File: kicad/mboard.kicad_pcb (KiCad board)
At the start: 2 copper layers, 66 x 48.3 mm, 3 parts

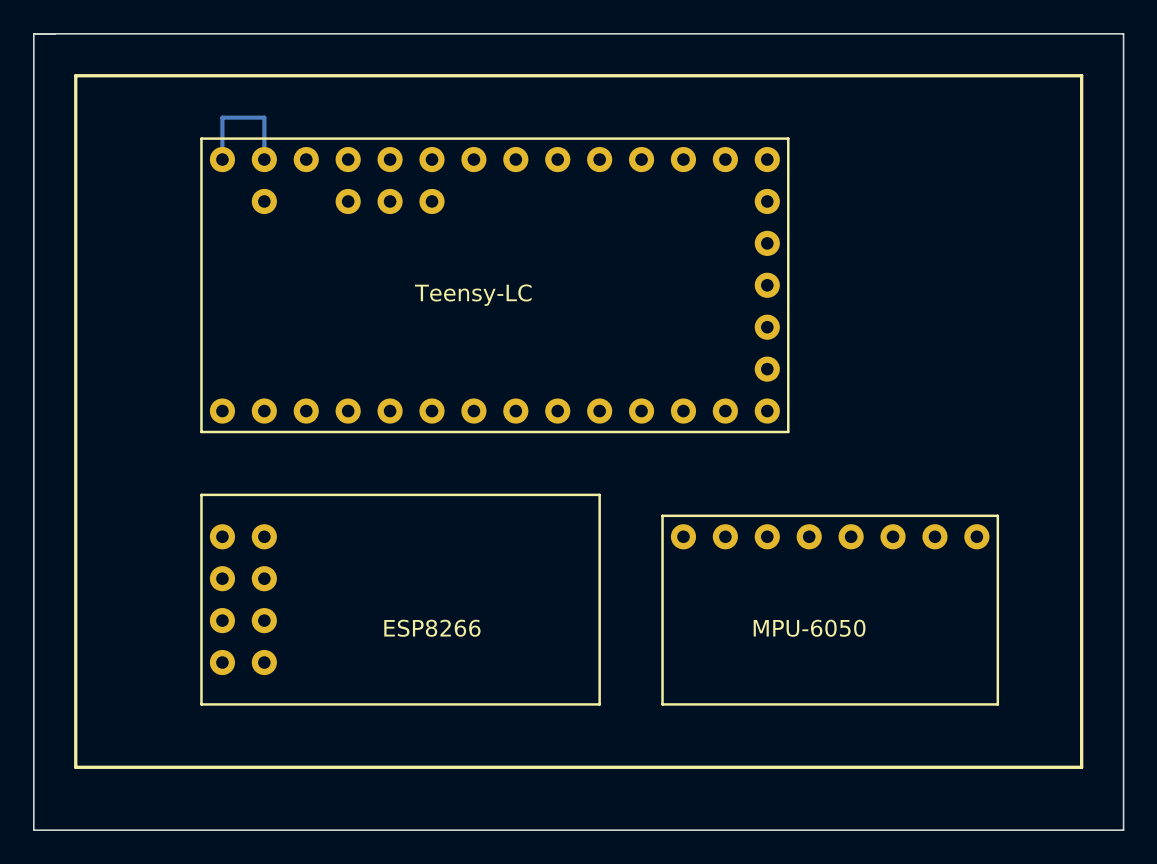
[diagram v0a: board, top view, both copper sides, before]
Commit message: mpu6050 thin
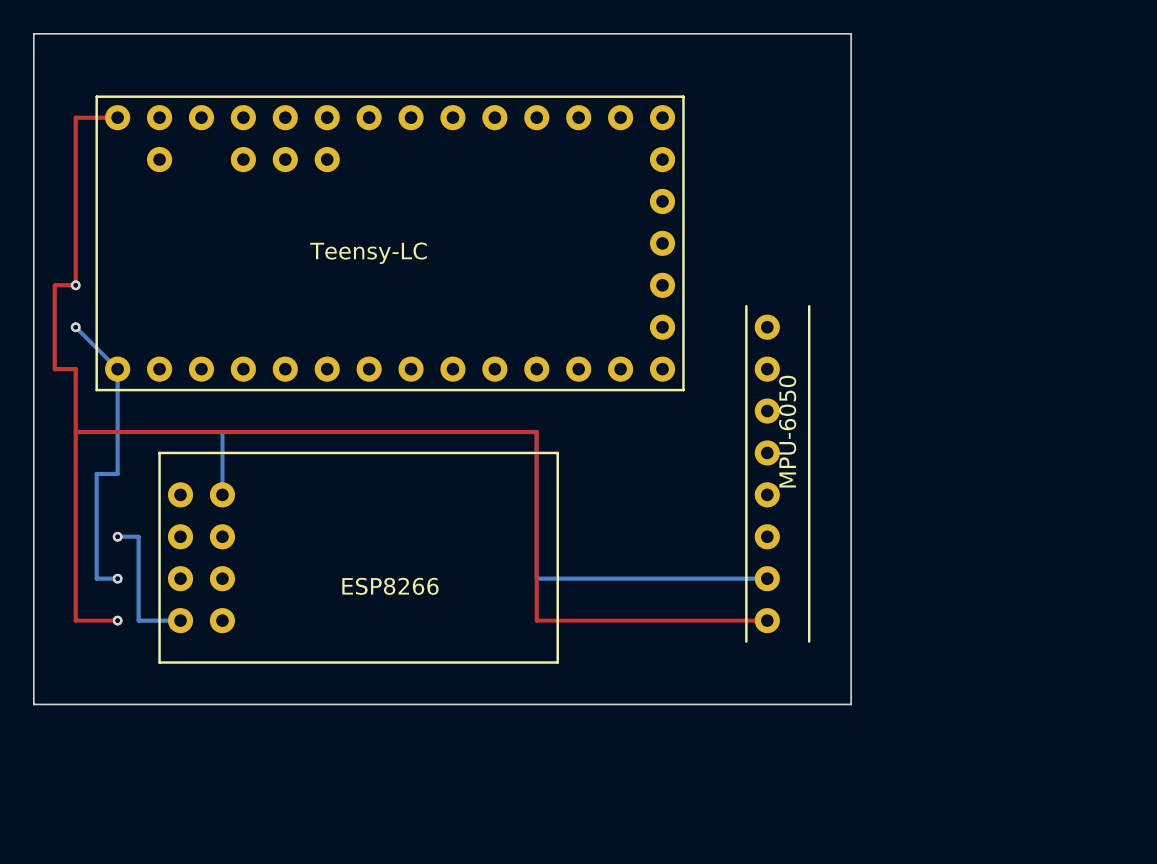
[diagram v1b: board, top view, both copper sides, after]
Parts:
- MPU-6050: footprint modules:MPU6050 -> modules:MPU6050-thin
- moved MPU-6050 8.03 mm to (74.9, 63.5), turned to 90 degrees
- moved Teensy-LC 6.84 mm to (45.7, 48.3)
- moved ESP8266 3.59 mm to (47.0, 68.6)
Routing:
- net (no net): track 7.62 -> 171.2 mm, vias 0 -> 5
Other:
- board size 66 x 48.3 mm -> 49.5 x 40.6 mm
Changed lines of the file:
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@@
     (links 0)
     (no_connects 0)
-    (area 25.349999 35.509999 91.490001 83.870001)
+    (area 25.349999 35.509999 74.980001 76.250001)
     (thickness 1.6)
-    (drawings 9)
-    (tracks 3)
+    (drawings 4)
+    (tracks 30)
     (zones 0)
     (modules 3)
@@
     (pad_to_mask_clearance 0)
     (aux_axis_origin 0 0)
-    (visible_elements FFFFFF7F)
+    (visible_elements FFFFF77F)
     (pcbplotparams
       (layerselection 0x010f0_80000001)
@@
   )
   (module modules:ESP8266 (layer F.Cu)
-    (at 49.53 71.12)
+    (at 46.99 68.58)
     (fp_text reference ESP8266 (at 0 0.5) (layer F.SilkS)
       (effects (font (size 1 1) (thickness 0.15)))
@@
     (pad 9 thru_hole circle (at -10.16 -5.08) (size 1.524 1.524) (drill 0.762) (layers *.Cu *.Mask F.SilkS))
   )
-  (module modules:MPU6050 (layer F.Cu)
-    (at 72.39 71.12)
-    (fp_text reference MPU-6050 (at 0 0.5) (layer F.SilkS)
-      (effects (font (size 1 1) (thickness 0.15)))
-    )
-    (fp_text value MPU6050 (at 0 -0.5) (layer F.Fab)
-      (effects (font (size 1 1) (thickness 0.15)))
-    )
-    (fp_line (start -8.89 -6.35) (end 11.43 -6.35) (layer F.SilkS) (width 0.15))
-    (fp_line (start 11.43 -6.35) (end 11.43 5.08) (layer F.SilkS) (width 0.15))
-    (fp_line (start 11.43 5.08) (end -8.89 5.08) (layer F.SilkS) (width 0.15))
-    (fp_line (start -8.89 5.08) (end -8.89 -6.35) (layer F.SilkS) (width 0.15))
-    (pad 1 thru_hole circle (at -7.62 -5.08) (size 1.524 1.524) (drill 0.762) (layers *.Cu *.Mask F.SilkS))
-    (pad 2 thru_hole circle (at -5.08 -5.08) (size 1.524 1.524) (drill 0.762) (layers *.Cu *.Mask F.SilkS))
-    (pad 3 thru_hole circle (at -2.54 -5.08) (size 1.524 1.524) (drill 0.762) (layers *.Cu *.Mask F.SilkS))
-    (pad 4 thru_hole circle (at 0 -5.08) (size 1.524 1.524) (drill 0.762) (layers *.Cu *.Mask F.SilkS))
-    (pad 5 thru_hole circle (at 2.54 -5.08) (size 1.524 1.524) (drill 0.762) (layers *.Cu *.Mask F.SilkS))
-    (pad 6 thru_hole circle (at 5.08 -5.08) (size 1.524 1.524) (drill 0.762) (layers *.Cu *.Mask F.SilkS))
-    (pad 7 thru_hole circle (at 7.62 -5.08) (size 1.524 1.524) (drill 0.762) (layers *.Cu *.Mask F.SilkS))
-    (pad 8 thru_hole circle (at 10.16 -5.08) (size 1.524 1.524) (drill 0.762) (layers *.Cu *.Mask F.SilkS))
-  )
   (module modules:Teensy-LC (layer F.Cu)
-    (at 52.07 50.8)
+    (at 45.72 48.26)
     (fp_text reference Teensy-LC (at 0 0.5) (layer F.SilkS)
       (effects (font (size 1 1) (thickness 0.15)))
@@
     (pad 4 thru_hole circle (at -2.54 -5.08) (size 1.524 1.524) (drill 0.762) (layers *.Cu *.Mask F.SilkS))
   )
-  (gr_line (start 25.4 35.56) (end 26.67 35.56) (angle 90) (layer Edge.Cuts) (width 0.1))
-  (gr_line (start 25.4 83.82) (end 25.4 35.56) (angle 90) (layer Edge.Cuts) (width 0.1))
-  (gr_line (start 91.44 83.82) (end 25.4 83.82) (angle 90) (layer Edge.Cuts) (width 0.1))
-  (gr_line (start 91.44 35.56) (end 91.44 83.82) (angle 90) (layer Edge.Cuts) (width 0.1))
-  (gr_line (start 25.4 35.56) (end 91.44 35.56) (angle 90) (layer Edge.Cuts) (width 0.1))
-  (gr_line (start 88.9 38.1) (end 27.94 38.1) (angle 90) (layer F.SilkS) (width 0.2))
-  (gr_line (start 88.9 80.01) (end 88.9 38.1) (angle 90) (layer F.SilkS) (width 0.2))
-  (gr_line (start 27.94 80.01) (end 88.9 80.01) (angle 90) (layer F.SilkS) (width 0.2))
-  (gr_line (start 27.94 38.1) (end 27.94 80.01) (angle 90) (layer F.SilkS) (width 0.2))
-  (segment (start 36.83 40.64) (end 39.37 40.64) (width 0.25) (layer B.Cu) (net 0))
-  (segment (start 39.37 40.64) (end 39.37 43.18) (width 0.25) (layer B.Cu) (net 0))
-  (segment (start 36.83 43.18) (end 36.83 40.64) (width 0.25) (layer B.Cu) (net 0))
+  (module modules:MPU6050-thin (layer F.Cu)
+    (at 74.93 63.5 90)
+    (fp_text reference MPU-6050 (at 3.81 -3.81 90) (layer F.SilkS)
+      (effects (font (size 1 1) (thickness 0.15)))
+    )
+    (fp_text value MPU6050 (at -5.08 -3.81 90) (layer F.Fab)
+      (effects (font (size 1 1) (thickness 0.15)))
+    )
+    (fp_line (start -8.89 -6.35) (end 11.43 -6.35) (layer F.SilkS) (width 0.15))
+    (fp_line (start 11.43 -2.54) (end -8.89 -2.54) (layer F.SilkS) (width 0.15))
+    (pad 1 thru_hole circle (at -7.62 -5.08 90) (size 1.524 1.524) (drill 0.762) (layers *.Cu *.Mask F.SilkS))
+    (pad 2 thru_hole circle (at -5.08 -5.08 90) (size 1.524 1.524) (drill 0.762) (layers *.Cu *.Mask F.SilkS))
+    (pad 3 thru_hole circle (at -2.54 -5.08 90) (size 1.524 1.524) (drill 0.762) (layers *.Cu *.Mask F.SilkS))
+    (pad 4 thru_hole circle (at 0 -5.08 90) (size 1.524 1.524) (drill 0.762) (layers *.Cu *.Mask F.SilkS))
+    (pad 5 thru_hole circle (at 2.54 -5.08 90) (size 1.524 1.524) (drill 0.762) (layers *.Cu *.Mask F.SilkS))
+    (pad 6 thru_hole circle (at 5.08 -5.08 90) (size 1.524 1.524) (drill 0.762) (layers *.Cu *.Mask F.SilkS))
+    (pad 7 thru_hole circle (at 7.62 -5.08 90) (size 1.524 1.524) (drill 0.762) (layers *.Cu *.Mask F.SilkS))
+    (pad 8 thru_hole circle (at 10.16 -5.08 90) (size 1.524 1.524) (drill 0.762) (layers *.Cu *.Mask F.SilkS))
+  )
+  (gr_line (start 74.93 76.2) (end 25.4 76.2) (angle 90) (layer Edge.Cuts) (width 0.1))
+  (gr_line (start 74.93 35.56) (end 74.93 76.2) (angle 90) (layer Edge.Cuts) (width 0.1))
+  (gr_line (start 25.4 35.56) (end 74.93 35.56) (angle 90) (layer Edge.Cuts) (width 0.1))
+  (gr_line (start 25.4 35.56) (end 25.4 76.2) (angle 90) (layer Edge.Cuts) (width 0.1))
+  (segment (start 31.75 66.04) (end 31.75 71.12) (width 0.25) (layer B.Cu) (net 0))
+  (segment (start 31.75 66.04) (end 30.48 66.04) (width 0.25) (layer B.Cu) (net 0))
+  (via (at 30.48 66.04) (size 0.6) (layers F.Cu B.Cu) (net 0))
+  (via (at 30.48 68.58) (size 0.6) (layers F.Cu B.Cu) (net 0))
+  (segment (start 29.21 68.58) (end 30.48 68.58) (width 0.25) (layer B.Cu) (net 0))
+  (segment (start 29.21 62.23) (end 29.21 68.58) (width 0.25) (layer B.Cu) (net 0))
+  (segment (start 34.29 71.12) (end 31.75 71.12) (width 0.25) (layer B.Cu) (net 0))
+  (via (at 30.48 71.12) (size 0.6) (layers F.Cu B.Cu) (net 0))
+  (segment (start 30.48 71.12) (end 27.94 71.12) (width 0.25) (layer F.Cu) (net 0))
+  (via (at 27.94 53.34) (size 0.6) (layers F.Cu B.Cu) (net 0))
+  (segment (start 27.94 53.34) (end 30.48 55.88) (width 0.25) (layer B.Cu) (net 0))
+  (segment (start 27.94 50.8) (end 26.67 50.8) (width 0.25) (layer F.Cu) (net 0))
+  (segment (start 30.48 40.64) (end 27.94 40.64) (width 0.25) (layer F.Cu) (net 0))
+  (segment (start 27.94 40.64) (end 27.94 50.8) (width 0.25) (layer F.Cu) (net 0))
+  (via (at 27.94 50.8) (size 0.6) (layers F.Cu B.Cu) (net 0))
+  (segment (start 27.94 55.88) (end 27.94 59.69) (width 0.25) (layer F.Cu) (net 0))
+  (segment (start 26.67 55.88) (end 27.94 55.88) (width 0.25) (layer F.Cu) (net 0))
+  (segment (start 26.67 50.8) (end 26.67 55.88) (width 0.25) (layer F.Cu) (net 0))
+  (segment (start 30.48 59.69) (end 30.48 62.23) (width 0.25) (layer B.Cu) (net 0))
+  (segment (start 30.48 62.23) (end 29.21 62.23) (width 0.25) (layer B.Cu) (net 0))
+  (segment (start 27.94 71.12) (end 27.94 59.69) (width 0.25) (layer F.Cu) (net 0))
+  (segment (start 36.83 59.69) (end 36.83 63.5) (width 0.25) (layer B.Cu) (net 0))
+  (segment (start 30.48 59.69) (end 36.83 59.69) (width 0.25) (layer B.Cu) (net 0))
+  (segment (start 36.83 59.69) (end 55.88 59.69) (width 0.25) (layer B.Cu) (net 0))
+  (segment (start 55.88 68.58) (end 69.85 68.58) (width 0.25) (layer B.Cu) (net 0))
+  (segment (start 55.88 59.69) (end 55.88 68.58) (width 0.25) (layer B.Cu) (net 0))
+  (segment (start 30.48 55.88) (end 30.48 59.69) (width 0.25) (layer B.Cu) (net 0))
+  (segment (start 27.94 59.69) (end 55.88 59.69) (width 0.25) (layer F.Cu) (net 0))
+  (segment (start 55.88 71.12) (end 69.85 71.12) (width 0.25) (layer F.Cu) (net 0))
+  (segment (start 55.88 59.69) (end 55.88 71.12) (width 0.25) (layer F.Cu) (net 0))
 )
